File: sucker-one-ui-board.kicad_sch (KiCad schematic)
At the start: 39 parts, among them J1 52271-1079, Q1 BSS138, SW1 LIFT, SW2 LOW, SW3 REVERSE, SW4 TRIGGER, SW5 DROP, SW6 HIGH, U1 WS2812-2020, U10 WS2812-2020, U11 WS2812-2020, U12 WS2812-2020, U2 WS2812-2020, U3 WS2812-2020, U4 WS2812-2020, U5 WS2812-2020, U6 WS2812-2020, U7 WS2812-2020, U8 WS2812-2020, U9 WS2812-2020

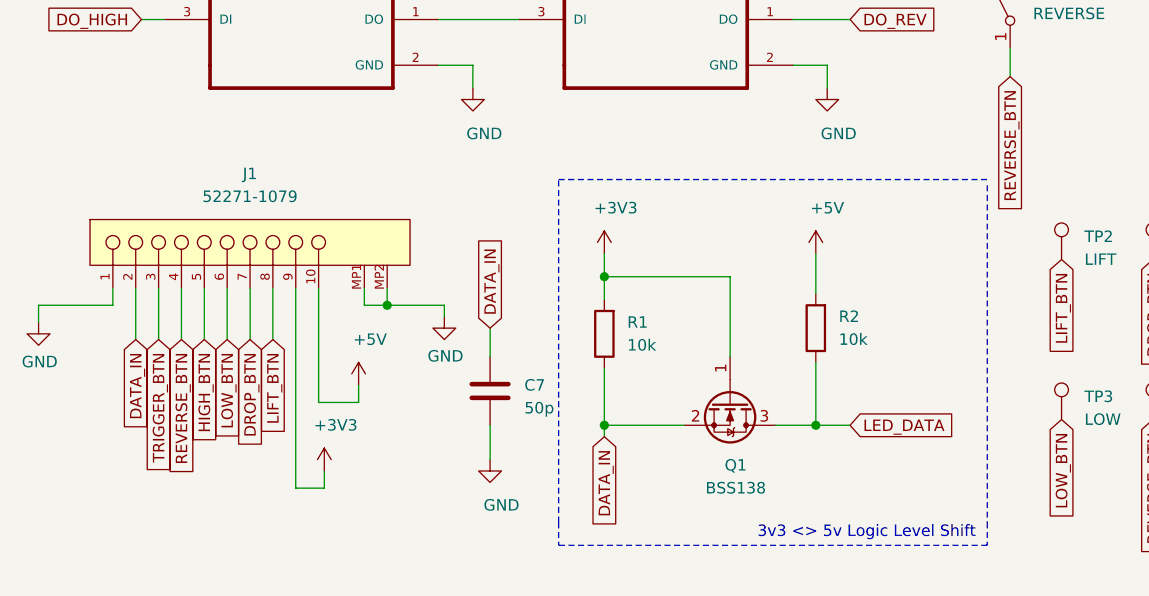
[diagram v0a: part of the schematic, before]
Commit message: Refactorings
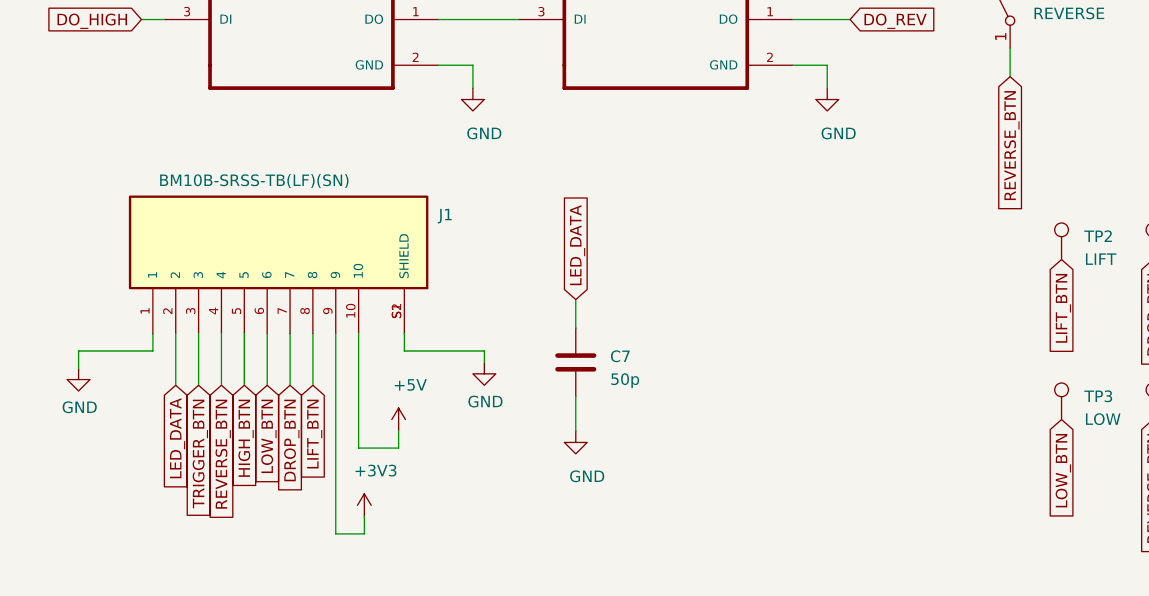
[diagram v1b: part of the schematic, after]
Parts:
- removed J1: 52271-1079, Molex-52271-1079-*:Molex-52271-1079-Manufacturer_Recommended, symbol MOLEX 10 Pin 1mm FFC con:52271-1079
- removed Q1: BSS138, Package_TO_SOT_SMD:SOT-23, symbol Transistor_FET:BSS138
- removed R1, R2: 10k, Resistor_SMD:R_0603_1608Metric, symbol Device:R
- added J1: BM10B-SRSS-TB(LF)(SN), BM10B-SRSS-TB(LF)(SN):BM10B-SRSS-TB(LF)(SN), symbol BM10B-SRSS-TB(LF)(SN):BM10B-SRSS-TB(LF)(SN)
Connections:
- net DATA_IN is gone; now on net LED_DATA: C7.1
- net +3V3: now also J1.9
- net +5V: now also J1.10
- net DROP_BTN: now also J1.7
- net GND: now also J1.1, J1.S1 (SHIELD), J1.S2 (SHIELD)
- net HIGH_BTN: now also J1.5
- net LED_DATA: now also J1.2
- net LIFT_BTN: now also J1.8
- net LOW_BTN: now also J1.6
- net REVERSE_BTN: now also J1.4
- net TRIGGER_BTN: now also J1.3
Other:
- note removed: "3v3 <> 5v Logic Level Shift"
- moved on the sheet: C7

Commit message: Cleanup and generate iBOM
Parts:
- TP1, TP10, TP2, TP3, TP4, TP5, TP6, TP7, TP8, TP9: now left out of the parts list
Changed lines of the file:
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@@
   )
   (symbol (lib_id "Connector:TestPoint") (at 128.905 162.56 0) (unit 1)
-    (in_bom yes) (on_board yes)
+    (in_bom no) (on_board yes)
     (property "Reference" "TP2" (id 0) (at 131.445 160.02 0)
       (effects (font (size 1.27 1.27)) (justify left))
@@
   )
   (symbol (lib_id "Connector:TestPoint") (at 128.905 180.34 0) (unit 1)
-    (in_bom yes) (on_board yes)
+    (in_bom no) (on_board yes)
     (property "Reference" "TP3" (id 0) (at 131.445 177.8 0)
       (effects (font (size 1.27 1.27)) (justify left))
@@
   )
   (symbol (lib_id "Connector:TestPoint") (at 139.065 162.56 0) (unit 1)
-    (in_bom yes) (on_board yes)
+    (in_bom no) (on_board yes)
     (property "Reference" "TP4" (id 0) (at 141.605 160.02 0)
       (effects (font (size 1.27 1.27)) (justify left))
@@
   )
   (symbol (lib_id "Connector:TestPoint") (at 139.065 180.34 0) (unit 1)
-    (in_bom yes) (on_board yes)
+    (in_bom no) (on_board yes)
     (property "Reference" "TP5" (id 0) (at 141.605 177.8 0)
       (effects (font (size 1.27 1.27)) (justify left))
@@
   )
   (symbol (lib_id "Connector:TestPoint") (at 152.4 162.56 0) (unit 1)
-    (in_bom yes) (on_board yes)
+    (in_bom no) (on_board yes)
     (property "Reference" "TP6" (id 0) (at 154.94 160.02 0)
       (effects (font (size 1.27 1.27)) (justify left))
@@
   )
   (symbol (lib_id "Connector:TestPoint") (at 152.4 180.34 0) (unit 1)
-    (in_bom yes) (on_board yes)
+    (in_bom no) (on_board yes)
     (property "Reference" "TP7" (id 0) (at 154.94 177.8 0)
       (effects (font (size 1.27 1.27)) (justify left))
@@
   )
   (symbol (lib_id "Connector:TestPoint") (at 166.37 162.56 0) (unit 1)
-    (in_bom yes) (on_board yes)
+    (in_bom no) (on_board yes)
     (property "Reference" "TP8" (id 0) (at 168.91 160.02 0)
       (effects (font (size 1.27 1.27)) (justify left))
@@
   )
   (symbol (lib_id "Connector:TestPoint") (at 166.37 180.34 0) (unit 1)
-    (in_bom yes) (on_board yes)
+    (in_bom no) (on_board yes)
     (property "Reference" "TP9" (id 0) (at 168.91 177.8 0)
       (effects (font (size 1.27 1.27)) (justify left))
@@
   )
   (symbol (lib_id "Connector:TestPoint") (at 258.445 149.225 0) (unit 1)
-    (in_bom yes) (on_board yes)
+    (in_bom no) (on_board yes)
     (property "Reference" "TP1" (id 0) (at 260.985 146.685 0)
       (effects (font (size 1.27 1.27)) (justify left))
@@
   )
   (symbol (lib_id "Connector:TestPoint") (at 265.43 125.095 0) (unit 1)
-    (in_bom yes) (on_board yes)
+    (in_bom no) (on_board yes)
     (property "Reference" "TP10" (id 0) (at 267.97 122.555 0)
       (effects (font (size 1.27 1.27)) (justify left))
